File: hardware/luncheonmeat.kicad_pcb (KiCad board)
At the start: 2 copper layers, 53 parts, among them J1 USB_B_Micro, J2 Conn_02x03_Odd_Even, Q1 Q_PMOS_DGS, Q2 Q_PMOS_DGS, Q3 Q_PMOS_DGS, SW1 SW_Push, SW10 7, SW11 4, SW12 1, SW13 *, SW2 9, SW3 6, SW4 3, SW5 #, SW6 8, SW7 5, SW8 2, SW9 0, U1 ATmega328PB-AU, U2 lsd100bag-101-20, U3 lsd100bag-101-20, U4 lsd100bag-101-20, U5 FT230XS, Y1 16MHz

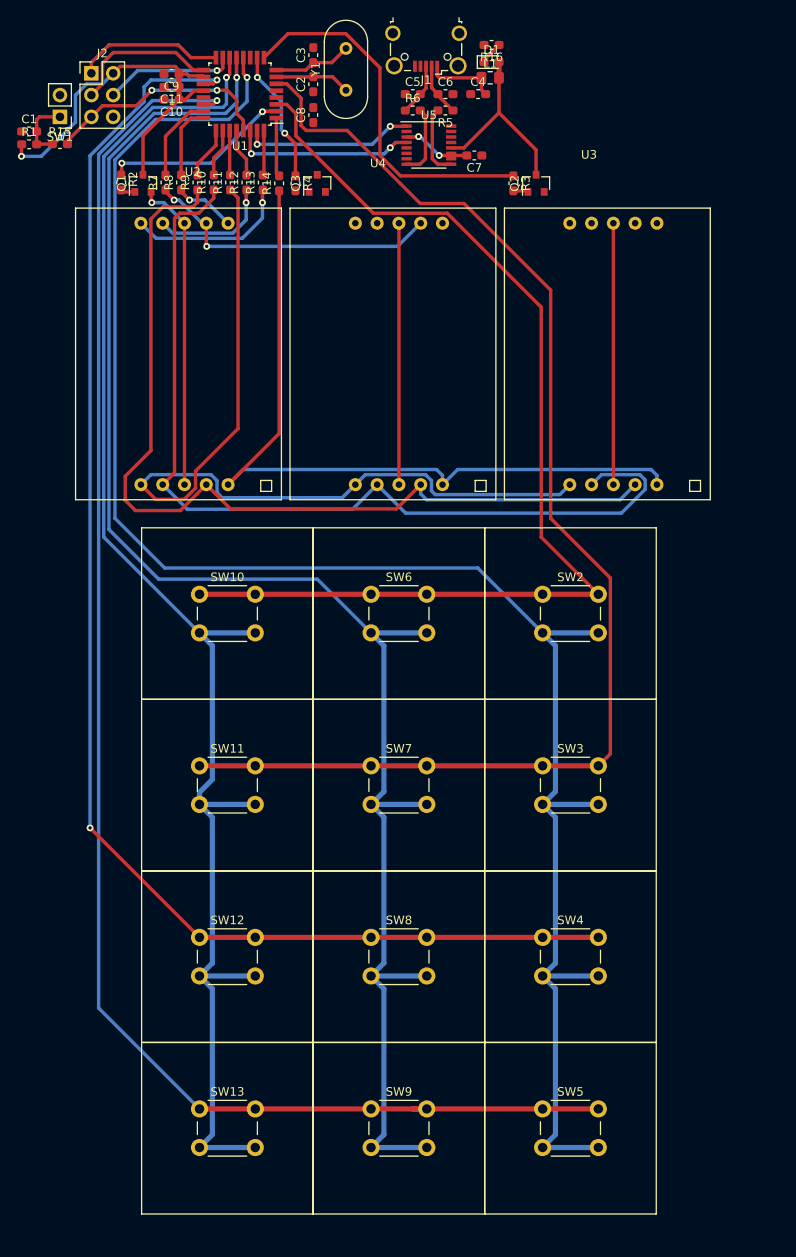
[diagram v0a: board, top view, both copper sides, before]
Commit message: Fix schematic, new board layout
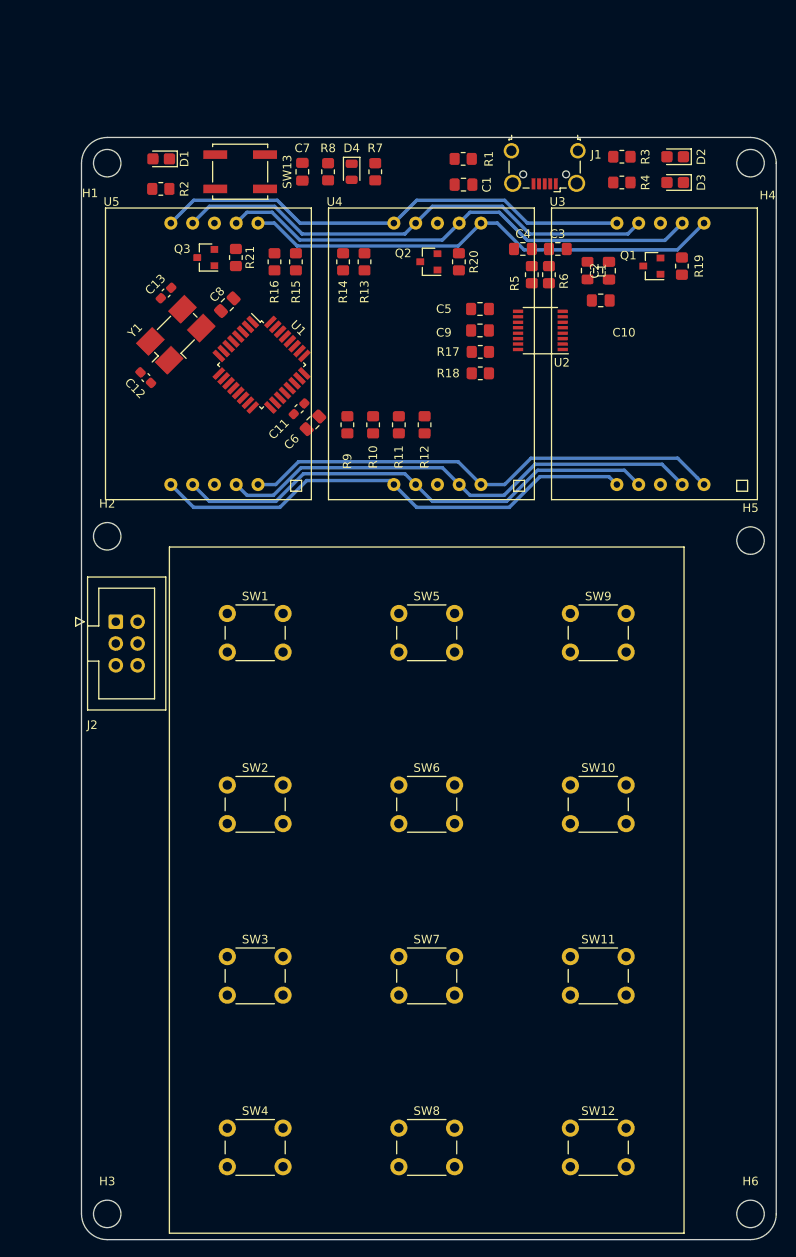
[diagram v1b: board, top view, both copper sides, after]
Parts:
- added C12: 22pF, Capacitor_SMD:C_0603_1608Metric_Pad1.08x0.95mm_HandSolder, F.Cu at (90.5, 92.5)
- added C13: 22pF, Capacitor_SMD:C_0603_1608Metric_Pad1.08x0.95mm_HandSolder, F.Cu at (92.9, 82.6)
- added D2: R, LED_SMD:LED_0805_2012Metric_Castellated, F.Cu at (152.2, 66.8)
- added D3: Y, LED_SMD:LED_0805_2012Metric_Castellated, F.Cu at (152.2, 69.8)
- added D4: D_Small, Diode_SMD:D_0805_2012Metric, F.Cu at (114.5, 68.5)
- added H1: MH, MountingHole:MountingHole_3.2mm_M3_DIN965, F.Cu at (86.0, 67.5)
- added H2: MH, MountingHole:MountingHole_3.2mm_M3_DIN965, F.Cu at (86.0, 111.0)
- added H3: MH, MountingHole:MountingHole_3.2mm_M3_DIN965, F.Cu at (86.0, 190.0)
- added H4: MH, MountingHole:MountingHole_3.2mm_M3_DIN965, F.Cu at (161.0, 67.5)
- added H5: MH, MountingHole:MountingHole_3.2mm_M3_DIN965, F.Cu at (161.0, 111.5)
- added H6: MH, MountingHole:MountingHole_3.2mm_M3_DIN965, F.Cu at (161.0, 190.0)
- added R17: 0R, Resistor_SMD:R_0805_2012Metric_Pad1.20x1.40mm_HandSolder, F.Cu at (129.5, 89.5)
- added R18: 0R, Resistor_SMD:R_0805_2012Metric_Pad1.20x1.40mm_HandSolder, F.Cu at (129.5, 92.0)
- added R19: 1k, Resistor_SMD:R_0805_2012Metric_Pad1.20x1.40mm_HandSolder, F.Cu at (153.0, 79.5)
- added R20: 1k, Resistor_SMD:R_0805_2012Metric_Pad1.20x1.40mm_HandSolder, F.Cu at (127.0, 79.0)
- added R21: 1k, Resistor_SMD:R_0805_2012Metric_Pad1.20x1.40mm_HandSolder, F.Cu at (101.0, 78.5)
- C1: value 100n -> 10nF; footprint Capacitor_SMD:C_0603_1608Metric_Pad1.05x0.95mm_HandSolder -> Capacitor_SMD:C_0805_2012Metric_Pad1.18x1.45mm_HandSolder
- C10, C7, C8, C9: value 100n -> 100nF; footprint Capacitor_SMD:C_0603_1608Metric_Pad1.05x0.95mm_HandSolder -> Capacitor_SMD:C_0805_2012Metric_Pad1.18x1.45mm_HandSolder
- C2: value 22p -> 10nF; footprint Capacitor_SMD:C_0603_1608Metric_Pad1.05x0.95mm_HandSolder -> Capacitor_SMD:C_0805_2012Metric_Pad1.18x1.45mm_HandSolder
- C3: value 22p -> 47p; footprint Capacitor_SMD:C_0603_1608Metric_Pad1.05x0.95mm_HandSolder -> Capacitor_SMD:C_0805_2012Metric_Pad1.18x1.45mm_HandSolder
- C4: value 10n -> 47p; footprint Capacitor_SMD:C_0603_1608Metric_Pad1.05x0.95mm_HandSolder -> Capacitor_SMD:C_0805_2012Metric_Pad1.18x1.45mm_HandSolder
- C5, C6: value 47p -> 100nF; footprint Capacitor_SMD:C_0603_1608Metric_Pad1.05x0.95mm_HandSolder -> Capacitor_SMD:C_0805_2012Metric_Pad1.18x1.45mm_HandSolder
- D1: value LED -> G; footprint Diode_SMD:D_0603_1608Metric_Pad1.05x0.95mm_HandSolder -> LED_SMD:LED_0805_2012Metric_Castellated
- J2: value Conn_02x03_Odd_Even -> AVR-ISP-6; footprint Connector_PinHeader_2.54mm:PinHeader_2x03_P2.54mm_Vertical -> Connector_IDC:IDC-Header_2x03_P2.54mm_Vertical
- R1: value 100k -> 1M; footprint Resistor_SMD:R_0603_1608Metric_Pad1.05x0.95mm_HandSolder -> Resistor_SMD:R_0805_2012Metric_Pad1.20x1.40mm_HandSolder
- R10, R11, R12, R13, R14, R15, R16, R5, R6, R7, R9: footprint Resistor_SMD:R_0603_1608Metric_Pad1.05x0.95mm_HandSolder -> Resistor_SMD:R_0805_2012Metric_Pad1.20x1.40mm_HandSolder
- R2: value 1k -> 300R; footprint Resistor_SMD:R_0603_1608Metric_Pad1.05x0.95mm_HandSolder -> Resistor_SMD:R_0805_2012Metric_Pad1.20x1.40mm_HandSolder
- R3, R4: value 1k -> 1.5k; footprint Resistor_SMD:R_0603_1608Metric_Pad1.05x0.95mm_HandSolder -> Resistor_SMD:R_0805_2012Metric_Pad1.20x1.40mm_HandSolder
- R8: value 300R -> 10k; footprint Resistor_SMD:R_0603_1608Metric_Pad1.05x0.95mm_HandSolder -> Resistor_SMD:R_0805_2012Metric_Pad1.20x1.40mm_HandSolder
- SW1: value SW_Push -> 7; footprint Connector_PinHeader_2.54mm:PinHeader_1x02_P2.54mm_Vertical -> Button_Switch_THT:SW_PUSH_6mm
- SW10: value 7 -> 6
- SW11: value 4 -> 3
- SW12: value 1 -> #
- SW13: value * -> SW_Push; footprint Button_Switch_THT:SW_PUSH_6mm -> Button_Switch_SMD:SW_Push_1P1T_NO_CK_KSC7xxJ
- SW2: value 9 -> 4
- SW3: value 6 -> 1
- SW4: value 3 -> *
- SW5: value # -> 8
- SW6: value 8 -> 5
- SW7: value 5 -> 2
- SW8: value 2 -> 0
- SW9: value 0 -> 9
- U2: value lsd100bag-101-20 -> FT230XS; footprint lsd100bag-101-20:lsd100bag-101-20 -> Package_SO:SSOP-16_3.9x4.9mm_P0.635mm
- U5: value FT230XS -> lsd100bag-101-20; footprint Package_SO:SSOP-16_3.9x4.9mm_P0.635mm -> lsd100bag-101-20:lsd100bag-101-20
- Y1: value 16MHz -> 8MHz; footprint Crystal:Crystal_HC49-4H_Vertical -> Crystal:Crystal_SMD_0603-4Pin_6.0x3.5mm_HandSoldering
- moved SW13 109.4 mm to (101.5, 68.5), turned to 180 degrees
- moved J2 64.0 mm to (87.0, 121.0)
- moved SW9 62.3 mm to (140.0, 120.0)
- moved SW1 61.1 mm to (100.0, 120.0), turned to 0 degrees
- moved SW5 60.1 mm to (120.0, 120.0)
- moved Q1 60.1 mm to (149.5, 79.5), turned to 180 degrees
- moved C10 55.2 mm to (143.5, 83.5), turned to 0 degrees
- moved C1 51.0 mm to (127.5, 70.0)
- moved R1 50.6 mm to (127.5, 67.0), turned to 180 degrees
- moved SW11 48.6 mm to (140.0, 160.0)
- moved SW12 48.6 mm to (140.0, 180.0)
- moved SW10 48.6 mm to (140.0, 140.0)
- moved C9 46.8 mm to (129.5, 87.0)
- moved SW2 43.0 mm to (100.0, 140.0)
- moved SW3 43.0 mm to (100.0, 160.0)
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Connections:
- C1 pad 1: Earth -> GND
- C10 pad 2: Earth -> GND
- C11 pad 2: Earth -> GND
- C2 pad 1: Earth -> GND
- C3 pad 1: Net-(C3-Pad1) -> GND
- C3 pad 2: Earth -> /D+
- C4 pad 1: Earth -> /D-
- C4 pad 2: Net-(C4-Pad2) -> GND
- C5 pad 1: Earth -> GND
- C5 pad 2: /D+ -> +5VD
- C6 pad 1: /D- -> GND
- C6 pad 2: Earth -> +5V
- C7 pad 1: Earth -> GND
- C8 pad 1: +5V -> GND
- C8 pad 2: Earth -> +5V
- C9 pad 2: Earth -> GND
- D1 pad 1: Net-(D1-Pad1) -> GND
- D1 pad 2: +5V -> Net-(D1-Pad2)
- J1 pad 1: Net-(C4-Pad2) -> Net-(C2-Pad2)
- J1 pad 5: Earth -> GND
- J1 pad 6: Net-(J1-Pad6) -> Net-(C1-Pad2)
- J2 pad 6: Earth -> GND
- L1 pad 1: Net-(C4-Pad2) -> Net-(C2-Pad2)
- R1 pad 1: +5V -> Net-(C1-Pad2)
- R1 pad 2: Net-(C1-Pad2) -> GND
- R11 pad 1: /SEG_E -> /SEG_C
- R12 pad 1: /SEG_F -> /SEG_RDP
- R13 pad 1: /SEG_G -> /SEG_F
- R14 pad 1: /SEG_RDP -> /SEG_G
- R15 pad 1: Net-(C1-Pad2) -> /SEG_B
- R15 pad 2: RESET -> Net-(R15-Pad2)
- R16 pad 1: Net-(D1-Pad1) -> /SEG_A
- R16 pad 2: Earth -> Net-(R16-Pad2)
- R2 pad 1: /SEG_SEL_0 -> Net-(D1-Pad2)
- R2 pad 2: Net-(Q1-Pad1) -> P_LED
- R3 pad 1: /SEG_SEL_1 -> Net-(D2-Pad2)
- R3 pad 2: Net-(Q2-Pad1) -> +5VD
- R4 pad 1: /SEG_SEL_2 -> Net-(D3-Pad2)
- R4 pad 2: Net-(Q3-Pad1) -> +5VD
- R7 pad 1: /SEG_A -> Net-(C7-Pad2)
- R7 pad 2: Net-(R7-Pad2) -> RESET
- R8 pad 1: /SEG_B -> Net-(C7-Pad2)
- R8 pad 2: Net-(R8-Pad2) -> +5V
- R9 pad 1: /SEG_C -> /SEG_E
- SW1 pad 1: Net-(C1-Pad2) -> /ROW_0
- SW1 pad 2: Earth -> /COL_2
- SW10 pad 1: /ROW_0 -> /ROW_1
- SW10 pad 2: /COL_2 -> /COL_0
- SW11 pad 1: /ROW_1 -> /ROW_2
- SW11 pad 2: /COL_2 -> /COL_0
- SW12 pad 1: /ROW_2 -> /ROW_3
- SW12 pad 2: /COL_2 -> /COL_0
- SW13 pad 1: /ROW_3 -> Net-(C7-Pad2)
- SW13 pad 2: /COL_2 -> GND
- SW2 pad 1: /ROW_0 -> /ROW_1
- SW2 pad 2: /COL_0 -> /COL_2
- SW3 pad 1: /ROW_1 -> /ROW_2
- SW3 pad 2: /COL_0 -> /COL_2
- SW4 pad 1: /ROW_2 -> /ROW_3
- SW4 pad 2: /COL_0 -> /COL_2
- SW5 pad 1: /ROW_3 -> /ROW_0
- SW5 pad 2: /COL_0 -> /COL_1
- SW6 pad 1: /ROW_0 -> /ROW_1
- SW7 pad 1: /ROW_1 -> /ROW_2
- SW8 pad 1: /ROW_2 -> /ROW_3
- SW9 pad 1: /ROW_3 -> /ROW_0
- SW9 pad 2: /COL_1 -> /COL_0
- U1 pad 1: Net-(R14-Pad2) -> Net-(R16-Pad2)
- U1 pad 11: Net-(U1-Pad11) -> P_LED
- U1 pad 21: Earth -> GND
- U1 pad 23: Net-(R7-Pad2) -> Net-(R9-Pad2)
- U1 pad 24: Net-(R8-Pad2) -> Net-(R10-Pad2)
- U1 pad 25: Net-(R9-Pad2) -> Net-(R11-Pad2)
- U1 pad 26: Net-(R10-Pad2) -> Net-(R12-Pad2)
- U1 pad 27: Net-(R11-Pad2) -> Net-(R13-Pad2)
- U1 pad 28: Net-(R12-Pad2) -> Net-(R14-Pad2)
- U1 pad 30: RX -> RXD
- U1 pad 31: TX -> TXD
- U1 pad 32: Net-(R13-Pad2) -> Net-(R15-Pad2)
- U1 pad 5: Earth -> GND
- U1 pad 7: Net-(C2-Pad2) -> Net-(C13-Pad1)
- U1 pad 8: Net-(C3-Pad1) -> Net-(C12-Pad2)
- U2 pad 1: /SEG_E -> TX_F
- U2 pad 10: /SEG_G -> +5VD
- U2 pad 2: /SEG_D -> Net-(U2-Pad2)
- U2 pad 3: Net-(Q1-Pad2) -> +5VD
- U2 pad 4: /SEG_C -> RX_F
- U2 pad 5: /SEG_RDP -> GND
- U2 pad 6: /SEG_B -> Net-(U2-Pad6)
- U2 pad 7: /SEG_A -> Net-(U2-Pad7)
- U2 pad 8: Net-(Q1-Pad2) -> /DR+
- U2 pad 9: /SEG_F -> /DR-
- U3 pad 3: Net-(Q2-Pad2) -> Net-(Q1-Pad2)
- U3 pad 8: Net-(Q2-Pad2) -> Net-(Q1-Pad2)
- U4 pad 3: Net-(Q3-Pad2) -> Net-(Q2-Pad2)
- U4 pad 8: Net-(Q3-Pad2) -> Net-(Q2-Pad2)
- U5 pad 1: TX -> /SEG_E
- U5 pad 10: Net-(C7-Pad2) -> /SEG_G
- U5 pad 2: Net-(U5-Pad2) -> /SEG_D
- U5 pad 3: Net-(C7-Pad2) -> Net-(Q3-Pad2)
- U5 pad 4: RX -> /SEG_C
- U5 pad 5: Earth -> /SEG_RDP
- U5 pad 6: Net-(U5-Pad6) -> /SEG_B
- U5 pad 7: Net-(U5-Pad7) -> /SEG_A
- U5 pad 8: /DR+ -> Net-(Q3-Pad2)
- U5 pad 9: /DR- -> /SEG_F
- Y1 pad 1: Net-(C2-Pad2) -> Net-(C12-Pad2)
- Y1 pad 2: Net-(C3-Pad1) -> GND
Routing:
- net /COL_0: track 210.4 -> 0.00 mm, vias 1 -> 0
- net /COL_1: track 191.4 -> 0.00 mm, vias 1 -> 0
- net /ROW_3: track 182.4 -> 0.00 mm, vias 1 -> 0
- net /COL_2: track 172.4 -> 0.00 mm, vias 1 -> 0
- net /ROW_2: track 164.1 -> 0.00 mm, vias 2 -> 0
- net /ROW_1: track 149.2 -> 0.00 mm
- net /ROW_0: track 124.9 -> 0.00 mm
- net +5V: track 68.6 -> 0.00 mm, vias 1 -> 0
- net /SEG_D: track 107.3 -> 57.7 mm
- net /SEG_C: track 107.3 -> 57.7 mm
- net /SEG_B: track 7.19 -> 56.8 mm, vias 1 -> 0
- net /SEG_SEL_1: track 43.1 -> 0.00 mm
- net /SEG_F: track 14.4 -> 57.3 mm, vias 1 -> 0
- net /SEG_E: track 100.5 -> 57.6 mm
- net /SEG_G: track 19.2 -> 56.4 mm, vias 1 -> 0
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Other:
- board outline added: 81 x 128.5 mm
- net class Default: clearance 0.2 -> 0.3; trace_width 0.25 -> 0.3; via_dia 0.8 -> 0.6
- net class Power added: clearance 0.5, trace_width 0.8, via_dia 0.9, via_drill 0.6
- net class Signals added: clearance 0.3, trace_width 0.3, via_dia 0.6, via_drill 0.4
- rule trace_clearance: 0.2 -> 0.3
